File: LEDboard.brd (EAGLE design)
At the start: 72 x 72 mm, 309 parts, among them IC1 REG1117, Q1 MMUN2133LT1G, U1 IS31FL3741_QFN60, U2 IS31FL3741_QFN60, U3 ATSAMD21G-A, U4 TPS61090RSAR, U5 MCP73831T-2ACI/OT

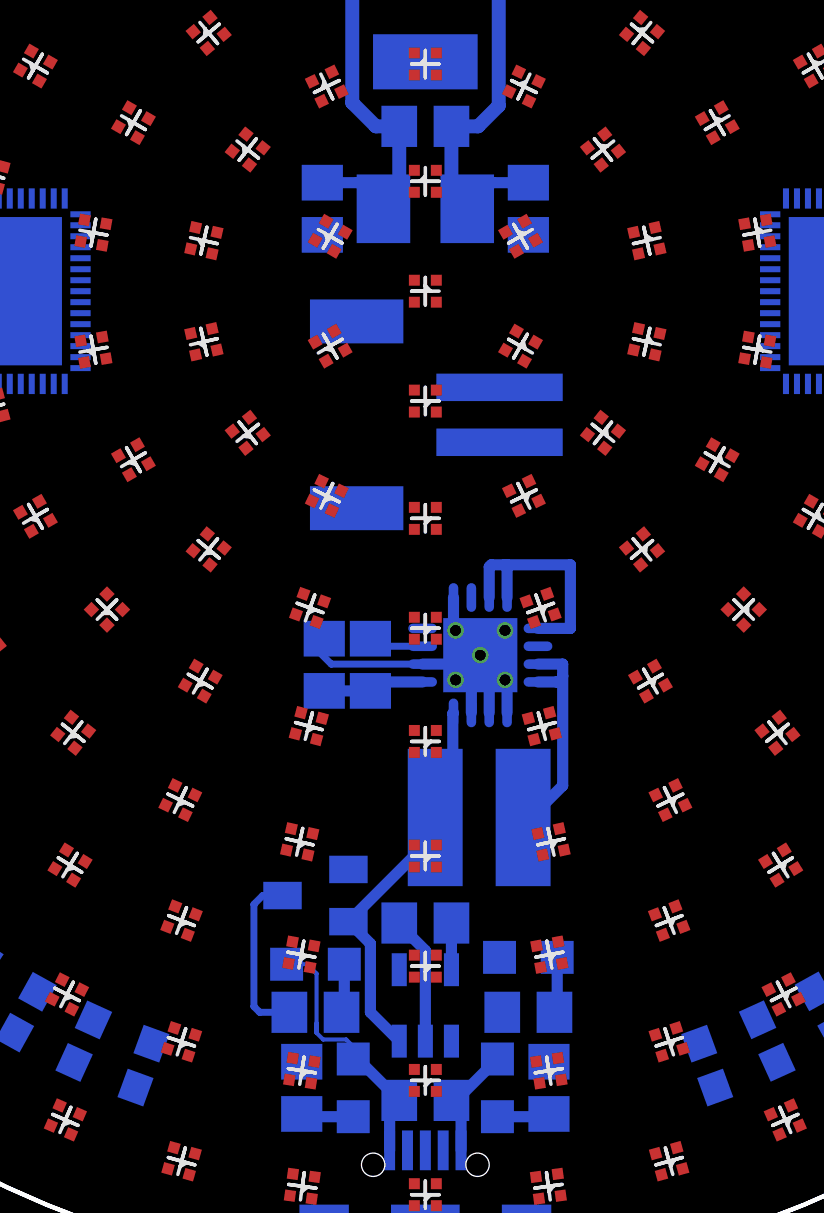
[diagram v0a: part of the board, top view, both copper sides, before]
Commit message: dear fucking god
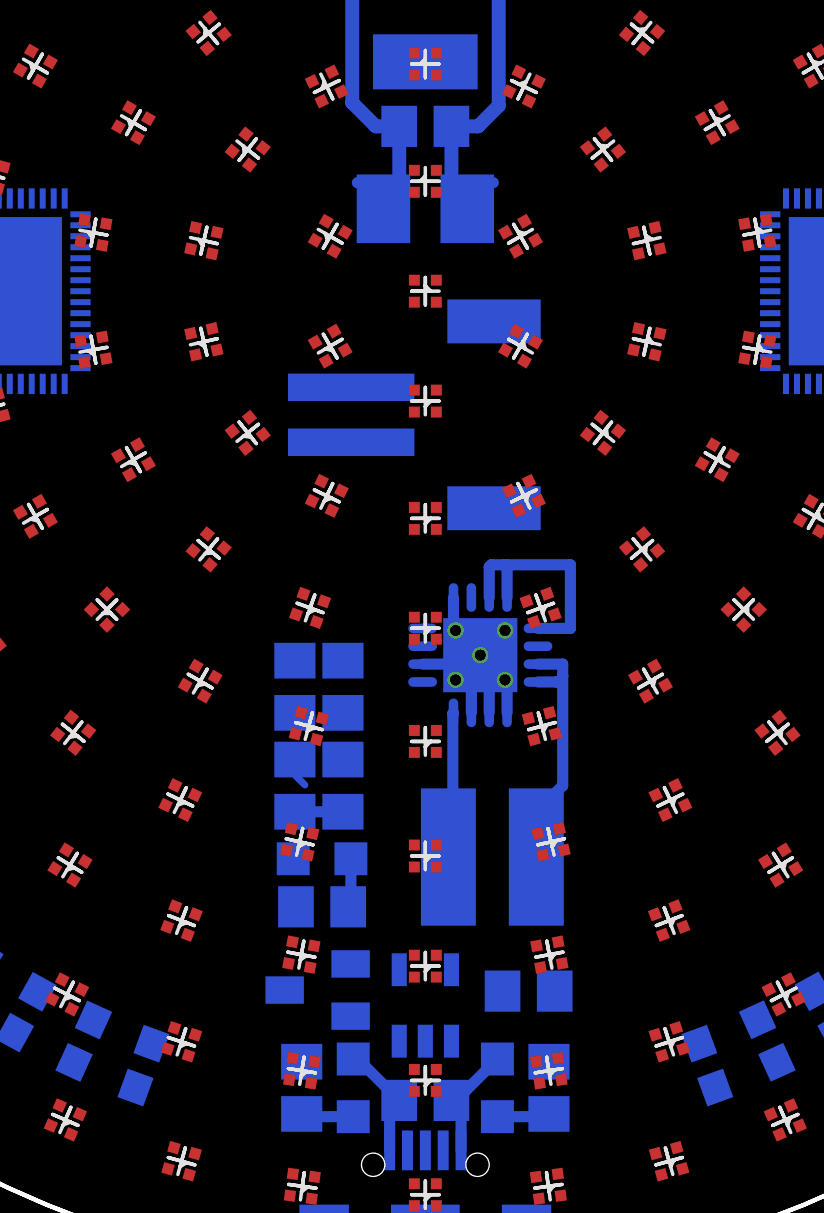
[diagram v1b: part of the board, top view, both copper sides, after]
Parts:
- removed PWR: BLUE, microbuilder:CHIPLED_0805_NOOUTLINE
- removed R77: 1K, microbuilder:0805-NO
- moved R79 18.7 mm to (-3.00, -14.4)
- moved R80 17.4 mm to (-4.75, -14.4), turned to 90 degrees
- moved R81 4.53 mm to (-4.75, -18.0)
- moved R82 4.51 mm to (-3.00, -18.0)
- moved R86 4.50 mm to (3.76, -25.5), turned to 180 degrees
- moved LBO 3.85 mm to (-3.76, -20.7)
- moved R83 3.85 mm to (-3.76, -22.4)
- moved Q1 3.44 mm to (-3.92, -25.4)
- moved B1 2.00 mm to (1.00, -4.50), turned to 90 degrees
- moved L1 1.52 mm to (2.44, -20.6)
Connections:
- removed net N$75: PWR.C, R77.1
- net 5.0V: no longer PWR.A
- net GND: no longer R77.2
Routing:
- net GND: track 47.1 -> 32.6 mm
- net VBAT: track 16.3 -> 6.38 mm
- net N$78: track 6.27 -> 0.00 mm
- net N$75: track 2.04 -> 0.00 mm
- net N$81: track 1.70 -> 0.00 mm
- net N$74: track 3.71 -> 2.24 mm
- net 5.0V: track 24.8 -> 23.5 mm
- net N$73: track 8.24 -> 9.31 mm
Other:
- board text removed: "PWR"
